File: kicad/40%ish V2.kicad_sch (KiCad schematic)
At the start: 92 parts, among them SW1 SW_Push, SW1-2 SW_Push, SW10 SW_Push, SW10-2 SW_Push, SW11 SW_Push, SW11-2 SW_Push, SW12 SW_Push, SW12-2 SW_Push, SW13 SW_Push, SW13-2 SW_Push, SW14 SW_Push, SW14-2 SW_Push, SW15 SW_Push, SW15-2 SW_Push, SW16 SW_Push, SW16-2 SW_Push, SW17 SW_Push, SW17-2 SW_Push, SW18 SW_Push, SW18-2 SW_Push, SW19 RotaryEncoder_Switch, SW2 SW_Push, SW2-2 SW_Push, SW20 SW_Push, SW20-2 SW_Push, SW3 SW_Push, SW3-2 SW_Push, SW4 SW_Push, SW4-2 SW_Push, SW5 SW_Push, SW5-2 SW_Push, SW6 SW_Push, SW6-2 SW_Push, SW7 SW_Push, SW7-2 SW_Push, SW8 SW_Push, SW8-2 SW_Push, SW9 SW_Push, SW9-2 SW_Push, U1 Nice_Nano_V2

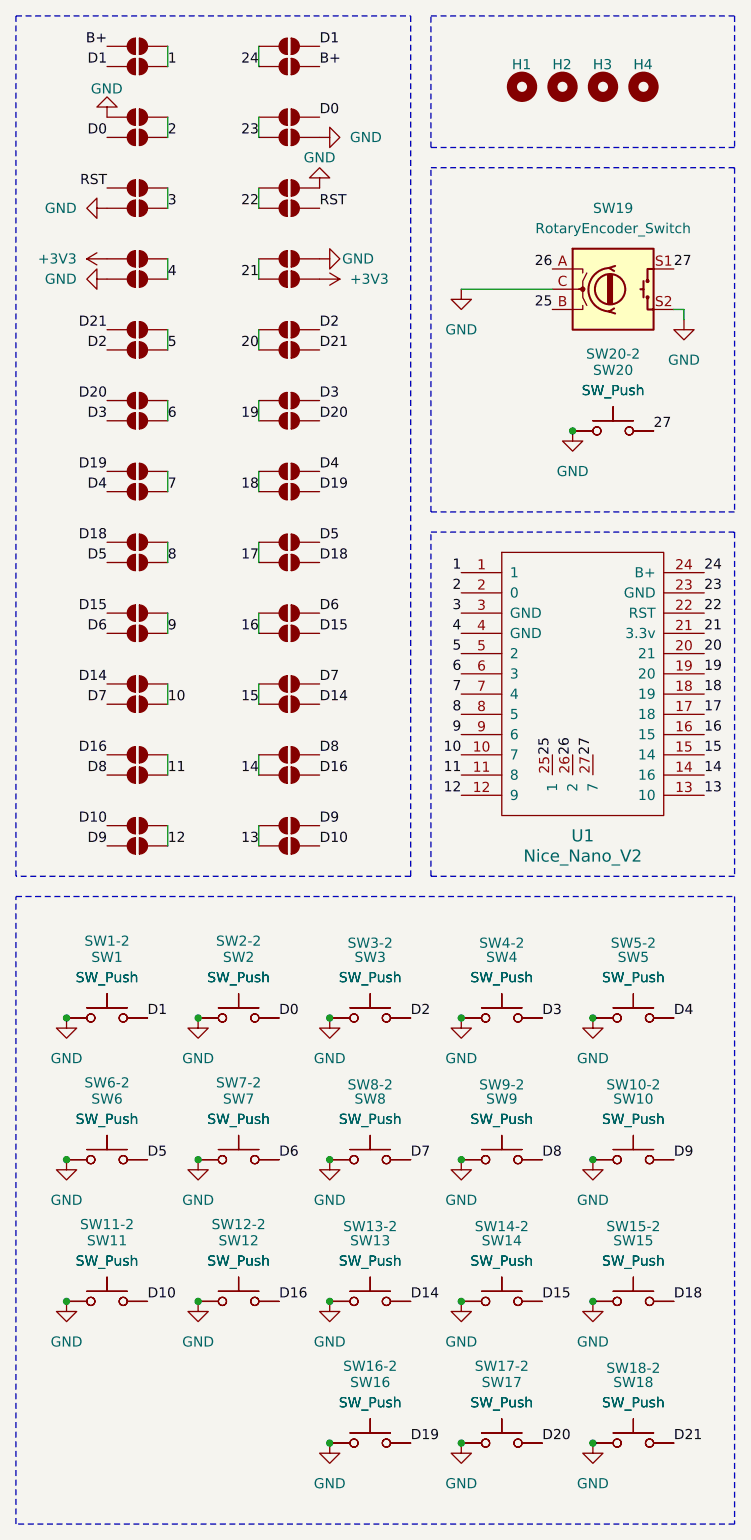
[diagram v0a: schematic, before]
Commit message: PCB done
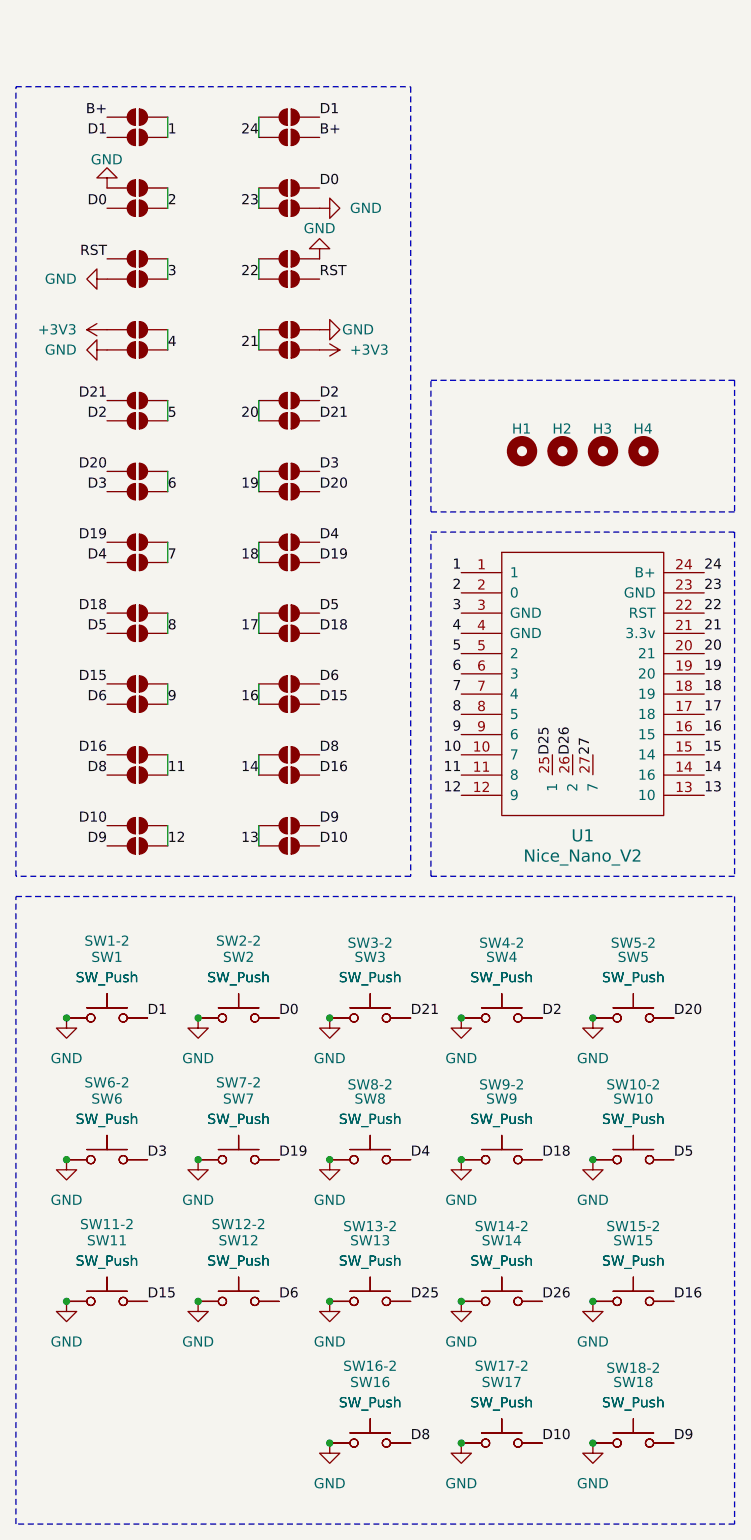
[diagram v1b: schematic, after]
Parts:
- removed JP31, JP32, JP43, JP44: SolderJumper_2_Open, Jumper:SolderJumper-2_P1.3mm_Open_TrianglePad1.0x1.5mm, symbol Jumper:SolderJumper_2_Open
- removed SW19: RotaryEncoder_Switch, Rotary_Encoder:RotaryEncoder_Alps_EC11E-Switch_Vertical_H20mm_CircularMountingHoles, symbol Device:RotaryEncoder_Switch
- removed SW20, SW20-2: SW_Push, MX_Hotswap:MX-Hotswap-1U, symbol Switch:SW_Push
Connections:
- net D14 is gone; now on net D25: SW13-2.2, SW13.2
- net D7 is gone; now on net D4: SW8-2.2, SW8.2
- net D10: now also SW17-2.2, SW17.2; no longer SW11-2.2, SW11.2
- net D15: now also SW11-2.2, SW11.2; no longer SW14-2.2, SW14.2
- net D16: now also SW15-2.2, SW15.2; no longer SW12-2.2, SW12.2
- net D18: now also SW9-2.2, SW9.2; no longer SW15-2.2, SW15.2
- net D19: now also SW7-2.2, SW7.2; no longer SW16-2.2, SW16.2
- net D2: now also SW4-2.2, SW4.2; no longer SW3-2.2, SW3.2
- net D20: now also SW5-2.2, SW5.2; no longer SW17-2.2, SW17.2
- net D21: now also SW3-2.2, SW3.2; no longer SW18-2.2, SW18.2
- net D3: now also SW6-2.2, SW6.2; no longer SW4-2.2, SW4.2
- net D4: no longer SW5-2.2, SW5.2
- net D5: now also SW10-2.2, SW10.2; no longer SW6-2.2, SW6.2
- net D6: now also SW12-2.2, SW12.2; no longer SW7-2.2, SW7.2
- net D8: now also SW16-2.2, SW16.2; no longer SW9-2.2, SW9.2
- net D9: now also SW18-2.2, SW18.2; no longer SW10-2.2, SW10.2
- net 25 renamed D25
- net 26 renamed D26
- net D26: now also SW14-2.2, SW14.2
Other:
- moved on the sheet: H1, H2, H3, H4

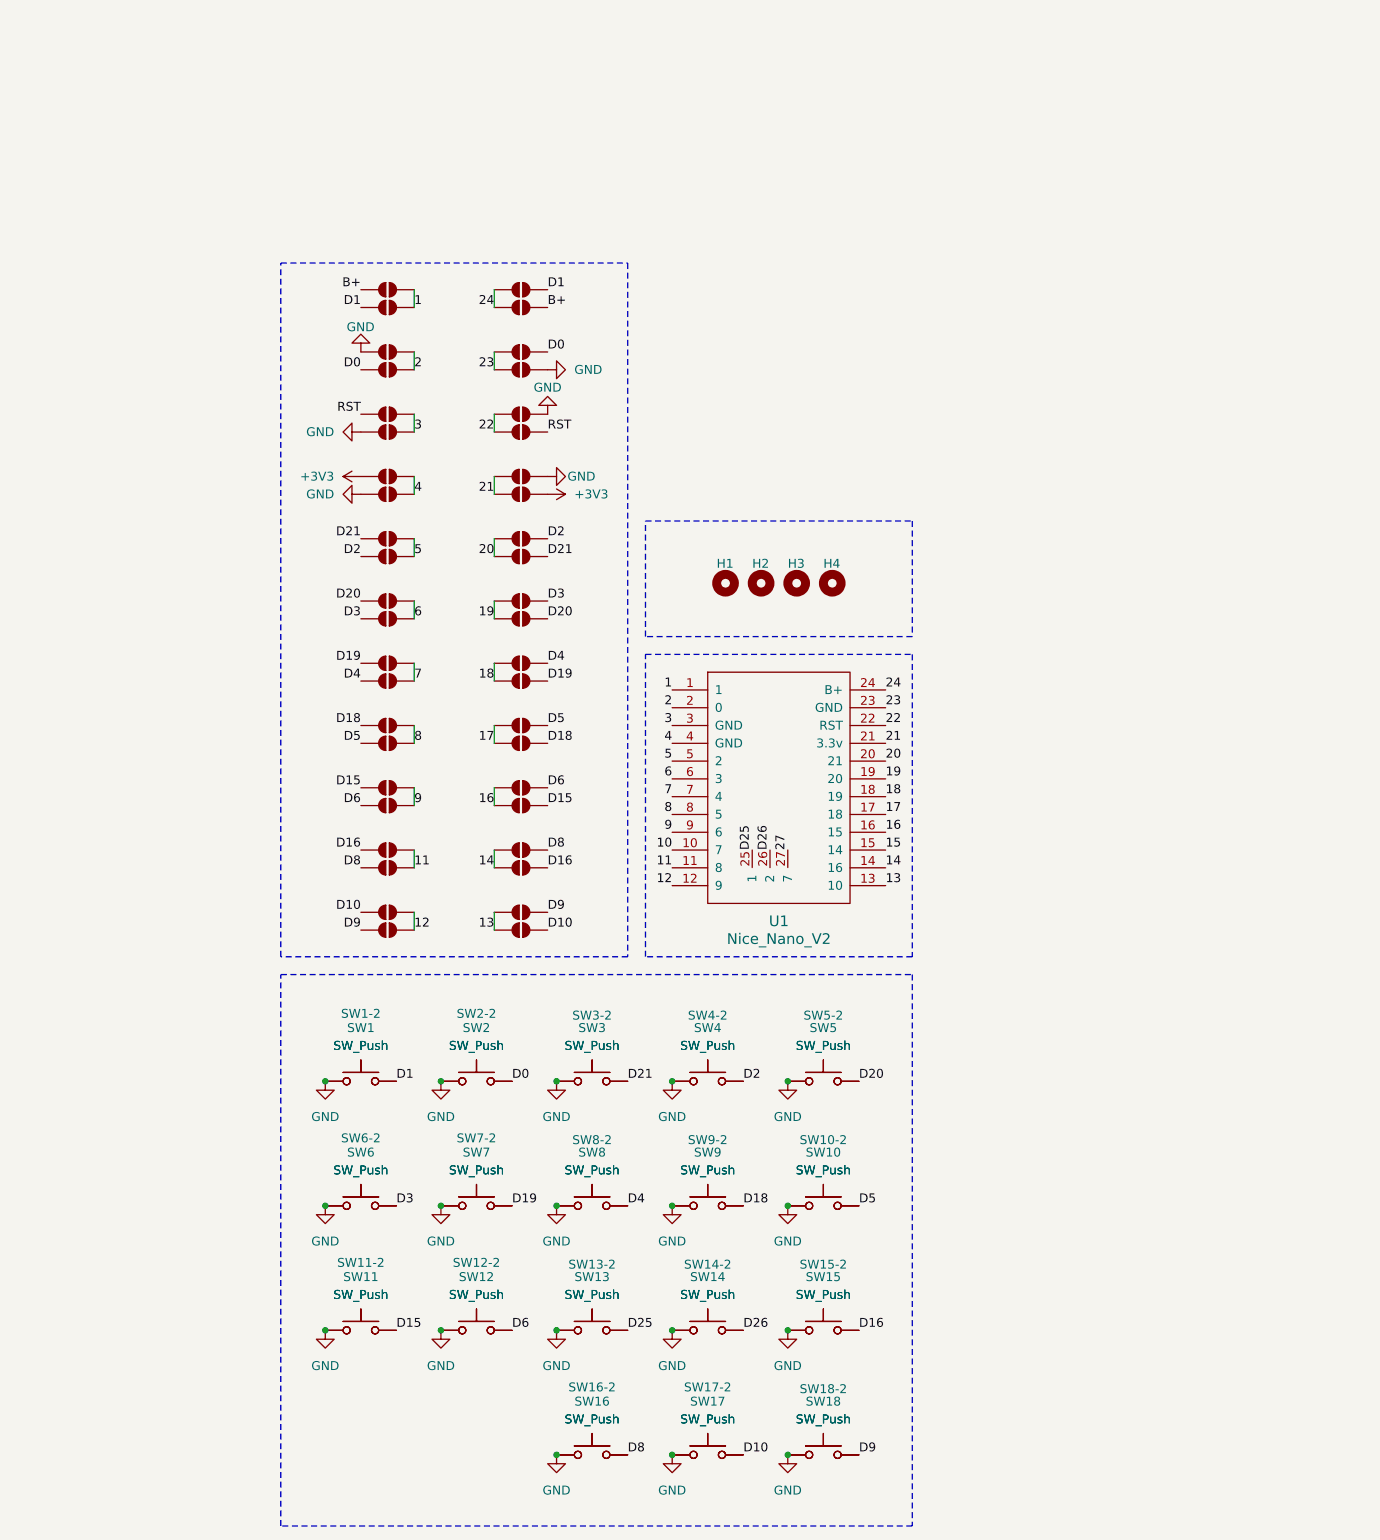
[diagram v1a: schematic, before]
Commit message: make 3D dir
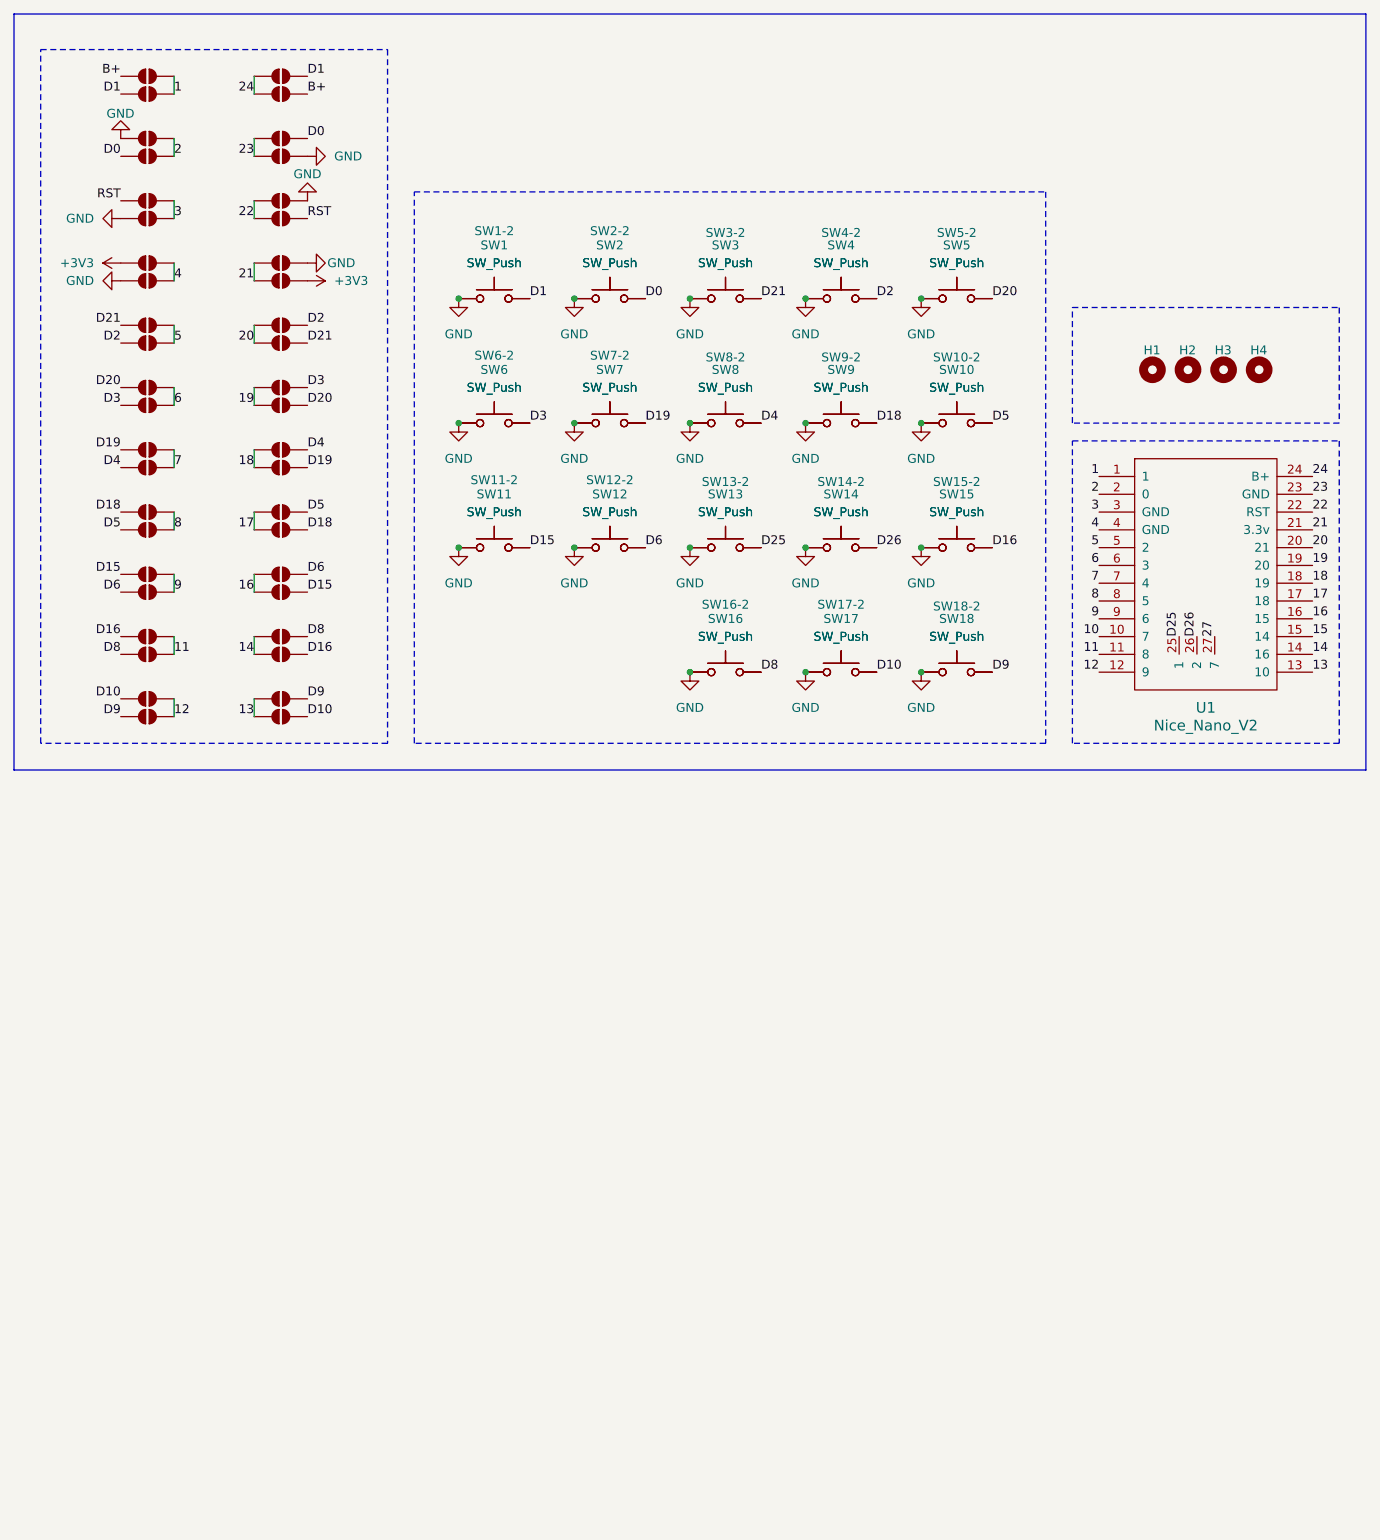
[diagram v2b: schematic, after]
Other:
- title: (none) -> 40%ish split keyboard 
- moved on the sheet: H1, H2, H3, H4, SW1, SW1-2, SW10, SW10-2, SW11, SW11-2, SW12, SW12-2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
